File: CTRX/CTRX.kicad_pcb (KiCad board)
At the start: 4 copper layers, 45 x 19 mm, 32 parts, among them J1 CON-SMA-EDGE-S, J3 Conn_02x05_Odd_Even, J4 USB-AM-S-X-X-TH, U1 nRF52820-QDxx, U2 NRF21540-QDAA-R7, U3 USBLC6-2SC6, U4 ME6211C33M5, Y1 32MHz

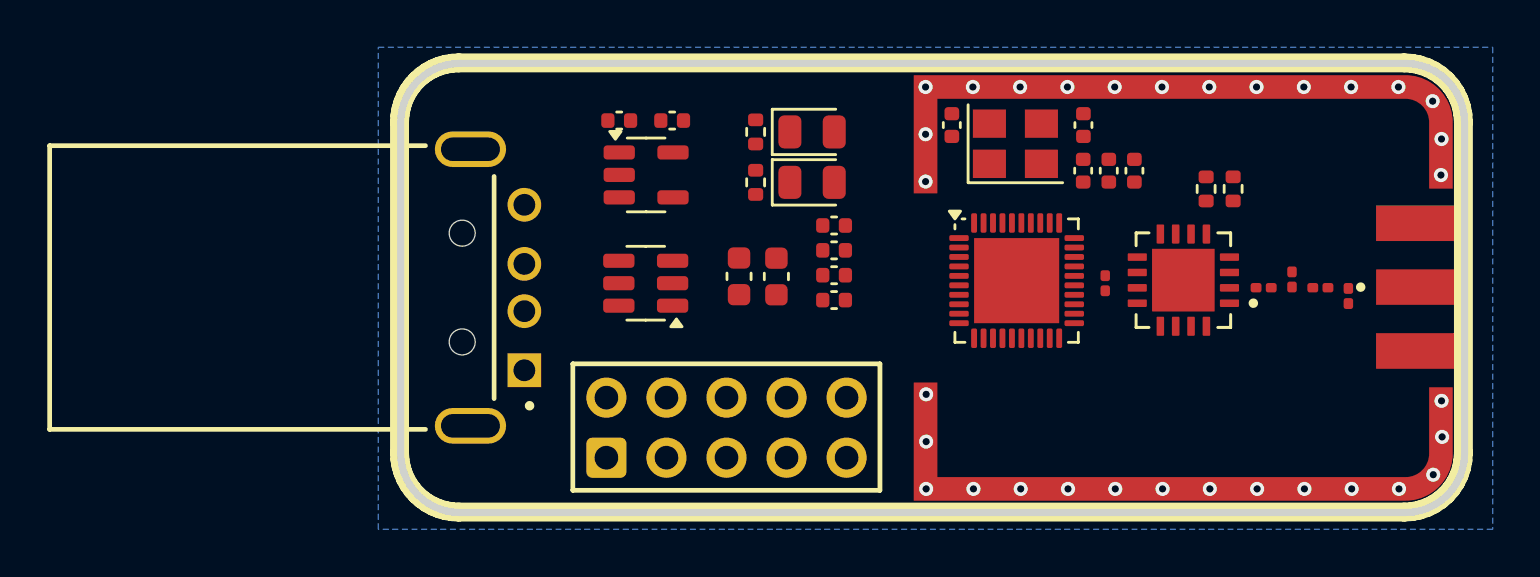
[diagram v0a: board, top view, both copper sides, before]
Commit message: ready
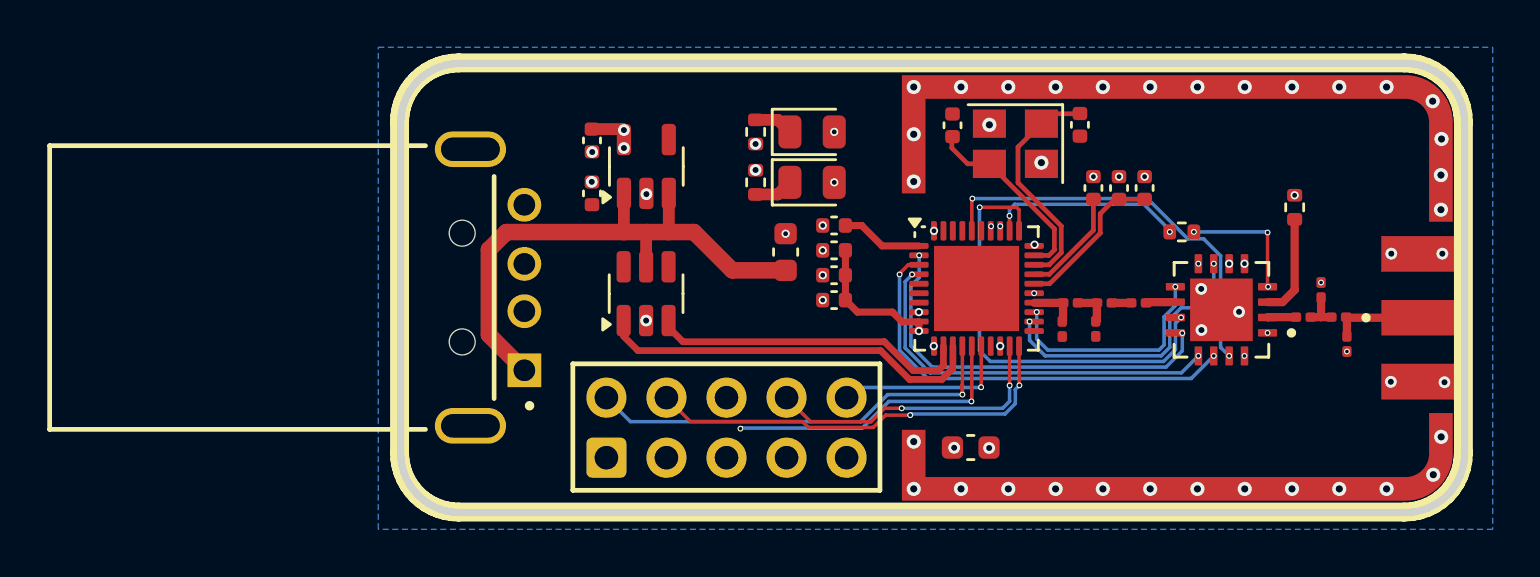
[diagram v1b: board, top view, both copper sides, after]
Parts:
- added C2: 1pF, Capacitor_SMD:C_0201_0603Metric, F.Cu at (142.5, 90.0)
- added C7: 1.2pF, Capacitor_SMD:C_0201_0603Metric, F.Cu at (143.9, 90.0)
- added L3: 4.7nH, Inductor_SMD:L_0201_0603Metric, F.Cu at (142.8, 88.9)
- added L4: 2.2nH, Inductor_SMD:L_0201_0603Metric, F.Cu at (144.3, 88.9)
- moved C6 12.2 mm to (138.6, 95.0), turned to 0 degrees
- moved C15 5.54 mm to (137.8, 81.4), turned to -90 degrees
- moved C12 5.42 mm to (143.2, 81.4), turned to 90 degrees
- moved C17 3.49 mm to (122.6, 82.1), turned to -90 degrees
- moved C16 3.29 mm to (122.6, 84.3), turned to -90 degrees
- moved R2 2.72 mm to (152.3, 84.9)
- moved L1 2.09 mm to (152.7, 89.5)
- moved R1 2.09 mm to (147.5, 85.9), turned to 0 degrees
- moved U2 2.04 mm to (149.2, 89.2)
- moved C11 2.03 mm to (154.5, 90.7)
- moved U1 1.73 mm to (138.9, 88.3)
- moved C18 1.64 mm to (145.7, 88.9), turned to 0 degrees
- moved L2 1.47 mm to (154.2, 89.5)
- moved J1 1.32 mm to (157.7, 89.6)
- moved C8 1.31 mm to (153.4, 88.4)
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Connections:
- U1 pad 24: NRF_ANT -> Net-(U1-ANT)
- U1 pad 9: +3.3V -> +5V
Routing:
- net +3.3V: track 0.50 -> 42.6 mm, vias 0 -> 8
- net +5V: track 0.00 -> 30.0 mm, vias 0 -> 1
- net NRF_PA_PDN: track 0.00 -> 18.8 mm, vias 0 -> 2
- net P014: track 0.00 -> 18.4 mm, vias 0 -> 1
- net NRF_SPI0_MISO: track 0.00 -> 18.4 mm, vias 0 -> 2
- net NRF_SWCLK: track 0.00 -> 18.2 mm, vias 0 -> 2
- net NRF_SPI0_CS: track 0.00 -> 17.3 mm, vias 0 -> 2
- net USB_D+: track 0.00 -> 17.2 mm
- net NRF_SPI0_SCK: track 0.00 -> 16.9 mm, vias 0 -> 2
- net NRF_SPI0_MOSI: track 0.00 -> 16.7 mm, vias 0 -> 2
- net P015: track 0.00 -> 14.2 mm, vias 0 -> 2
- net USB_D-: track 0.00 -> 14.0 mm
- net NRF_SWDIO: track 0.00 -> 12.6 mm, vias 0 -> 2
- net NRF_PA_RX_EN: track 0.00 -> 12.0 mm, vias 0 -> 2
- net NRF_LED1: track 0.00 -> 10.2 mm, vias 0 -> 2
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
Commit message: CTRX Order Ready
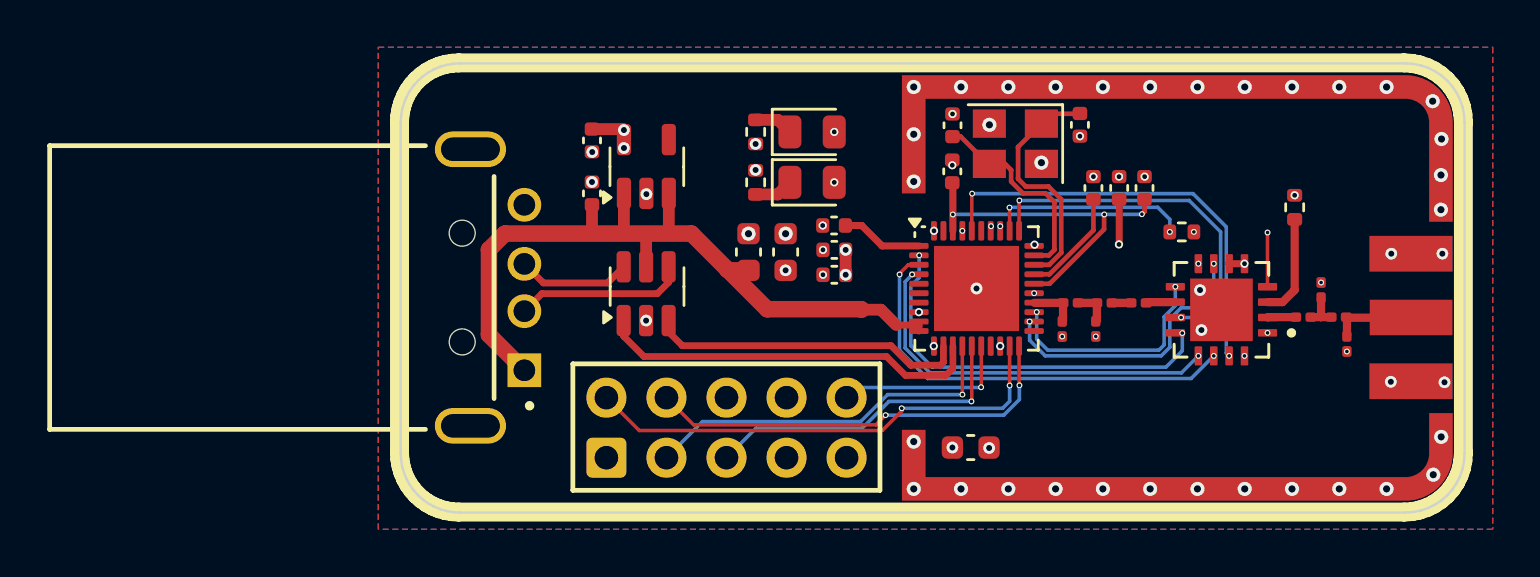
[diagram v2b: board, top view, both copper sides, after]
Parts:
- added C19: 4.7uF, Capacitor_SMD:C_0603_1608Metric, F.Cu at (129.2, 86.8)
- moved C4 12.3 mm to (144.9, 84.1), turned to 90 degrees
- moved C13 8.17 mm to (137.8, 83.4)
- moved C14 1.08 mm to (146.0, 84.1)
- moved C1 1.07 mm to (132.8, 86.7)
- moved C5 1.07 mm to (132.8, 87.7)
- moved J1 0.50 mm to (157.2, 89.5)
- turned U3 to 0 degrees
- turned U4 to 0 degrees
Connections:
- C1 pad 2: +5V -> +3.3V
- C3 pad 1: +5V -> +3.3V
- C4 pad 1: +5V -> +3.3V
- C5 pad 1: +5V -> +3.3V
- J3 pad 2: P014 -> NRF_SWDIO
- J3 pad 3: GND -> P014
- J3 pad 5: GND -> P015
- J3 pad 6: P015 -> unconnected-(J3-Pin_6-Pad6)
- J3 pad 8: NRF_SWDIO -> unconnected-(J3-Pin_8-Pad8)
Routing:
- net DEC4: track 6.63 -> 15.3 mm, vias 0 -> 3
- net NRF_SWDIO: track 12.6 -> 20.5 mm
- net USB_CONN_D-: track 0.00 -> 7.27 mm
- net USB_CONN_D+: track 0.52 -> 5.34 mm
- net NRF_PA_PDN: track 18.8 -> 15.3 mm
- net +3.3V: track 42.6 -> 45.5 mm, vias 8 -> 11
- net +5V: track 30.0 -> 32.8 mm, vias 1 -> 0
- net P014: track 18.4 -> 15.7 mm
- net NRF_SPI0_CS: track 17.3 -> 18.4 mm
- net NRF_XC2: track 8.09 -> 8.75 mm
- net NRF_XC1: track 9.94 -> 10.5 mm
- net P015: track 14.2 -> 13.7 mm, vias 2 -> 1
- net Net-(U2-MODE): track 5.42 -> 5.46 mm, vias 3 -> 2
- net GND: track 0.25 -> 0.22 mm, vias 62 -> 68
- added copper zone on F.Cu, net GND

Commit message: ready to order.
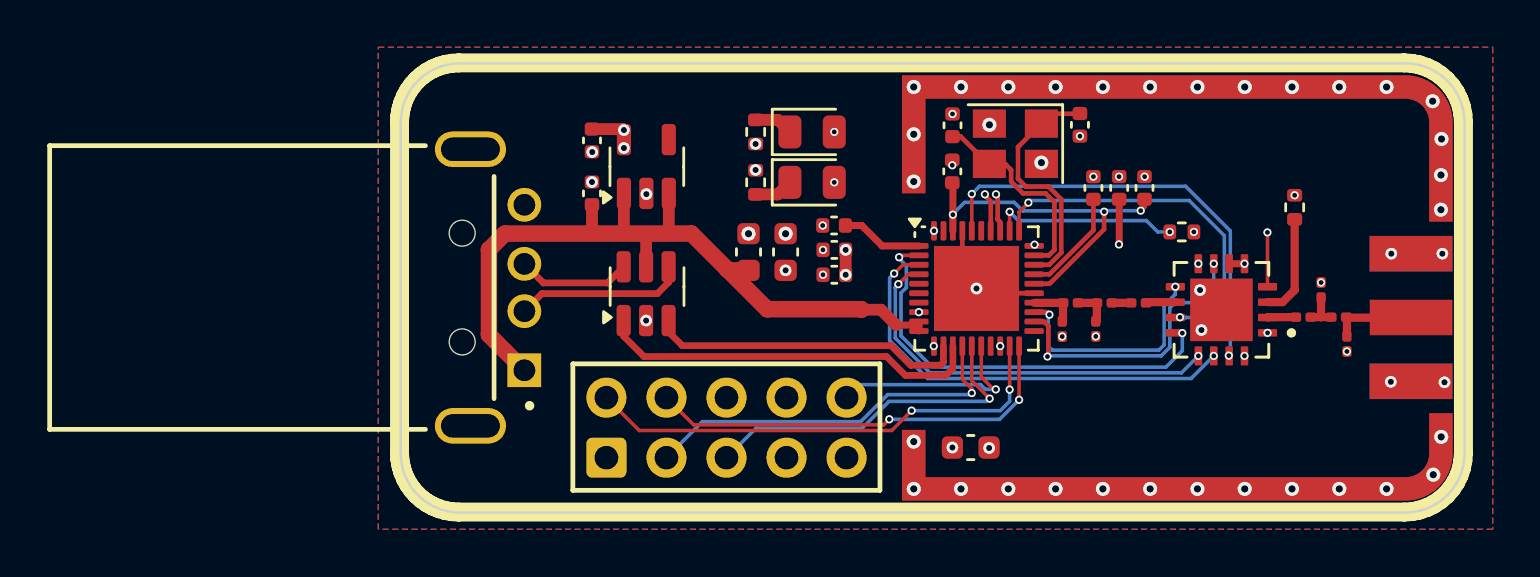
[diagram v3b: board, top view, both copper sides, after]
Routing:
- net GND: track 0.22 -> 5.43 mm, vias 68 -> 66
- net NRF_NRST: track 7.62 -> 8.76 mm
- net NRF_SPI0_SCK: track 16.9 -> 17.9 mm
- net P015: track 13.7 -> 14.7 mm
- net NRF_SPI0_MOSI: track 16.7 -> 17.4 mm
- net NRF_PA_TX_EN: track 9.47 -> 10.2 mm
- net P014: track 15.7 -> 16.3 mm
- net NRF_PA_MODE: track 8.51 -> 7.93 mm
